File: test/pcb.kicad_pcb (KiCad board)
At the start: 2 copper layers, 98 x 120 mm, 25 parts, among them M1 RasPiPico, SW1 SW_Push, SW10 SW_Push, SW11 SW_Push, SW12 SW_Push, SW13 SW_Push, SW14 SW_Push, SW15 SW_Push, SW16 SW_Push, SW17 SW_Push, SW18 SW_Push, SW19 SW_Push, SW2 SW_Push, SW20 SW_Push, SW21 SW_Push, SW22 SW_Push, SW3 SW_Push, SW4 SW_Push, SW5 SW_Push, SW7 SW_Push, SW8 SW_Push, SW9 SW_Push

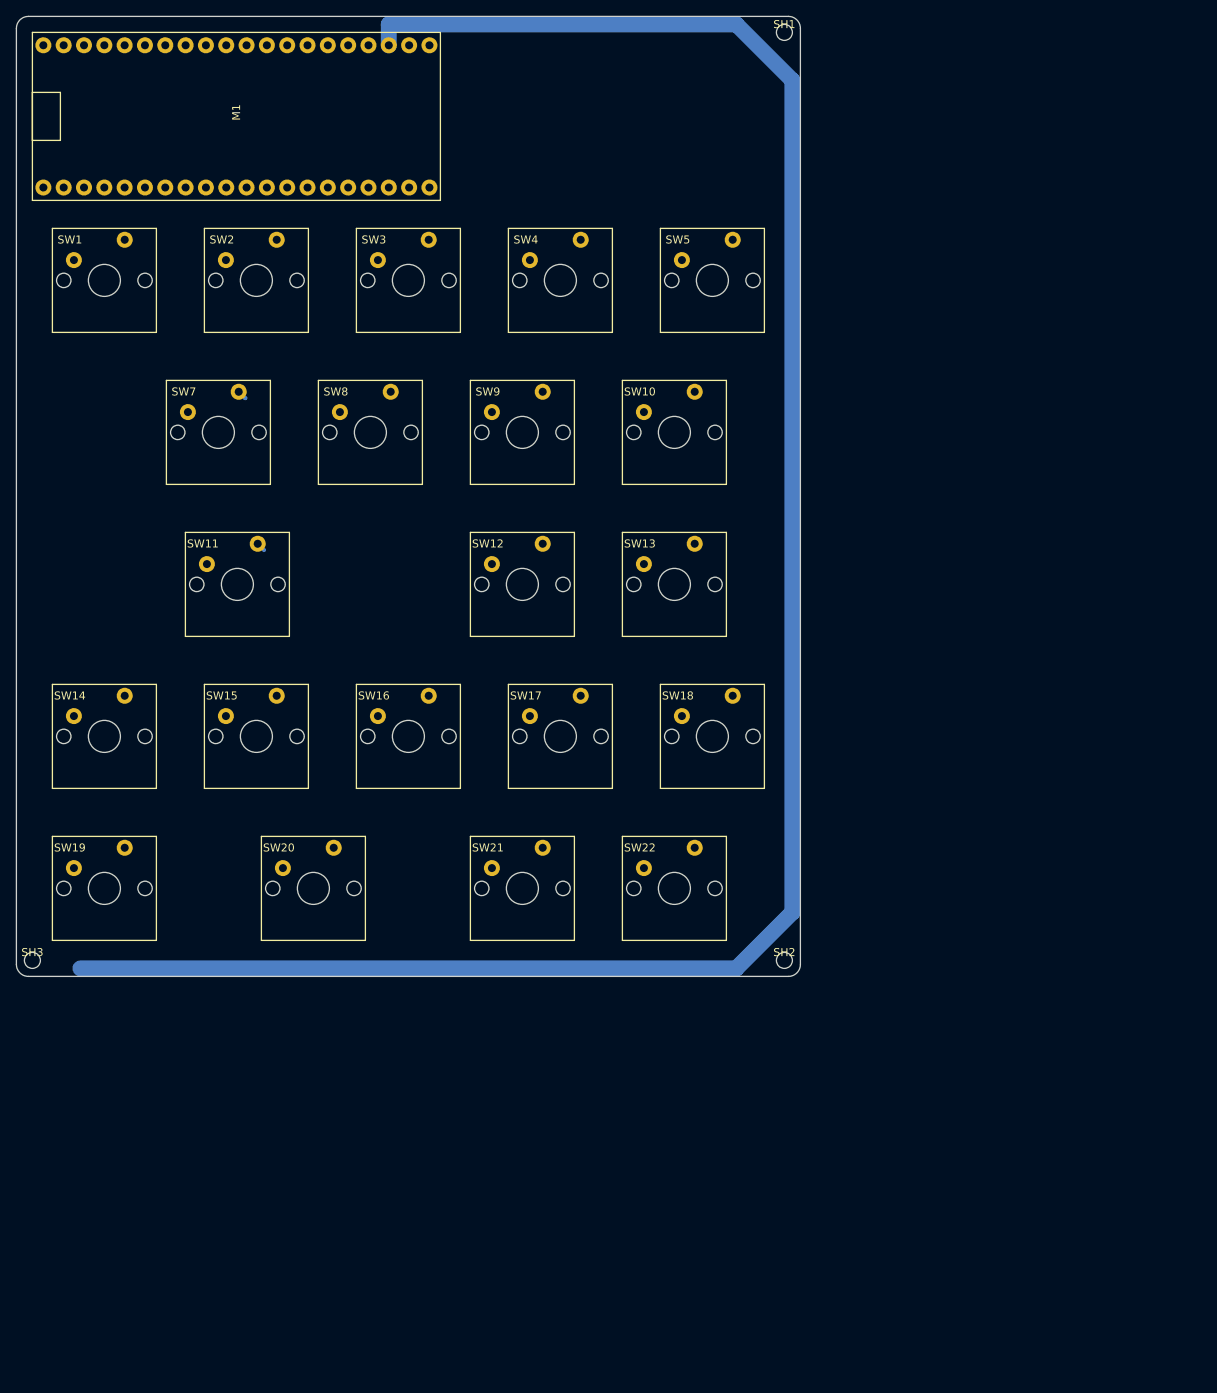
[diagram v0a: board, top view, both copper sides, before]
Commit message: fix file size 0
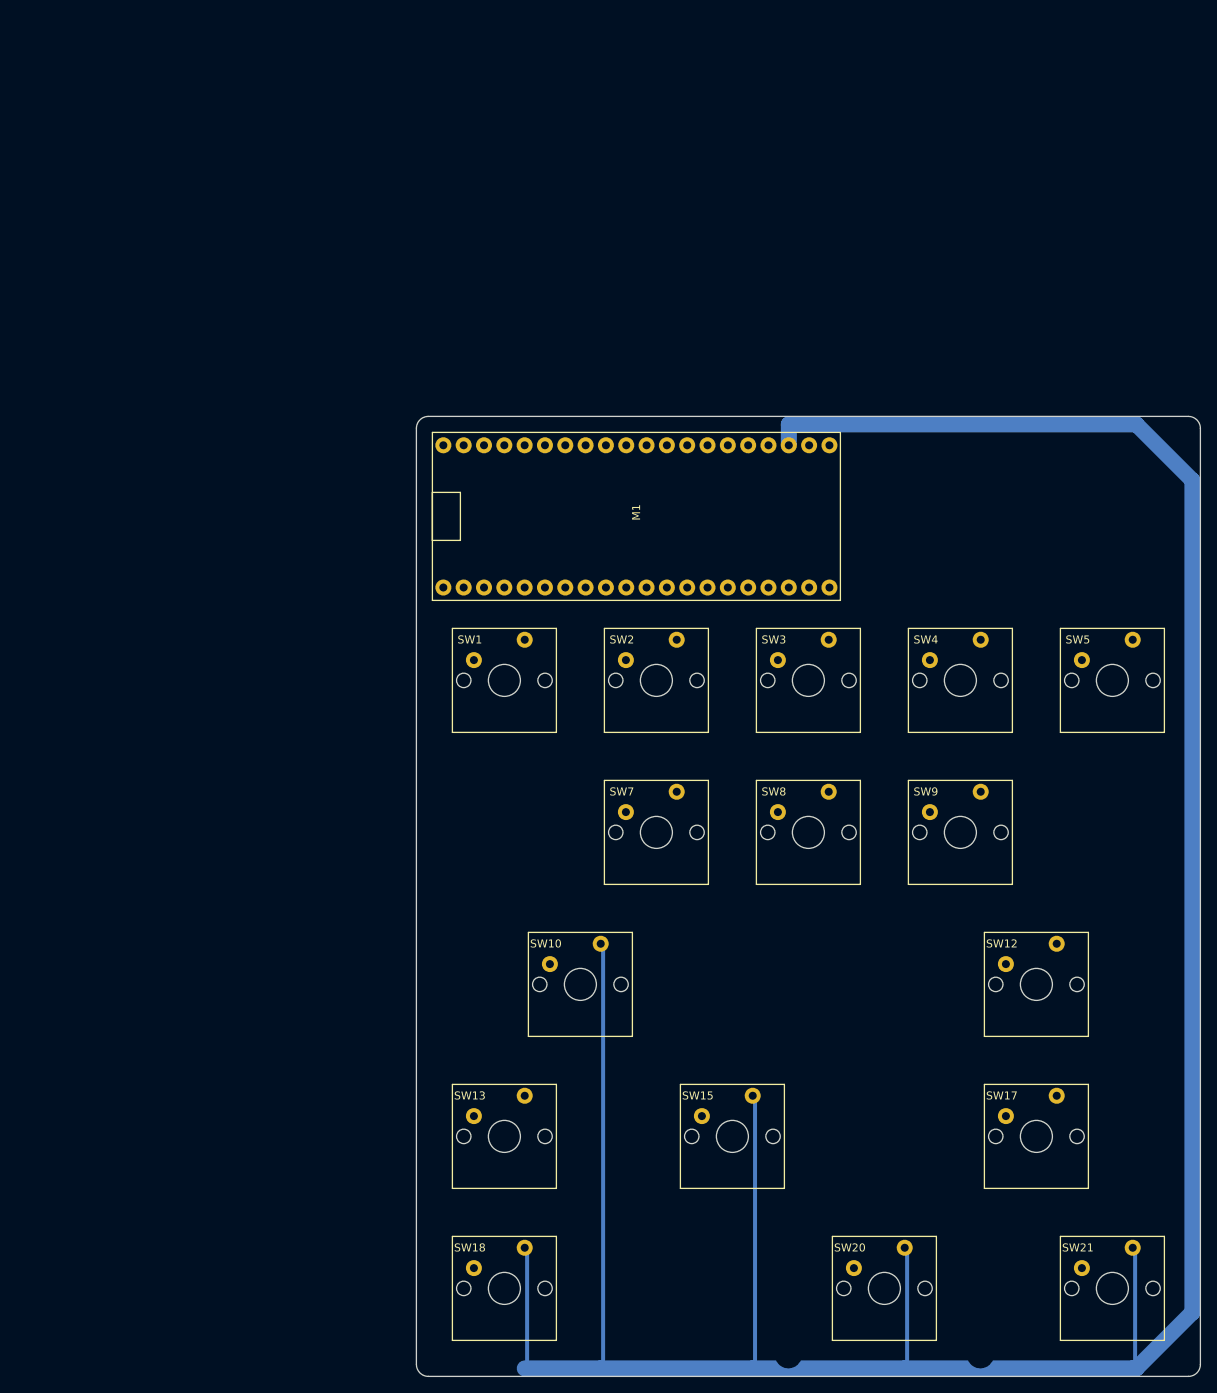
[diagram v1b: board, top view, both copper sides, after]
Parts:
- removed the M1 at (27.5, 12.5)
- removed SH2, SH3: SCREW_HOLE, footprint:screwhole
- removed SW11: SW_Push, footprint:keyswitch-with-stabilizer
- removed SW14, SW16, SW19, SW22: SW_Push, footprint:keyswitch
- M1: renamed from SH1; value SCREW_HOLE -> RasPiPico; footprint footprint:screwhole -> footprint:pipico
- SW10, SW20: footprint footprint:keyswitch -> footprint:keyswitch-with-stabilizer
- moved SW21 89.1 mm to (137.0, 159.0)
- moved SW20 87.1 mm to (108.5, 159.0)
- moved SW12 81.4 mm to (127.5, 121.0)
- moved SW15 77.7 mm to (89.5, 140.0)
- moved SW17 77.7 mm to (127.5, 140.0)
- moved SW7 74.1 mm to (80.0, 102.0)
- moved SW8 74.1 mm to (99.0, 102.0)
- moved SW9 74.1 mm to (118.0, 102.0)
- moved SW18 73.7 mm to (61.0, 159.0)
- moved SW13 72.2 mm to (61.0, 140.0)
- moved SW1 70.7 mm to (61.0, 83.0)
- moved SW2 70.7 mm to (80.0, 83.0)
- moved SW3 70.7 mm to (99.0, 83.0)
- moved SW4 70.7 mm to (118.0, 83.0)
- moved SW5 70.7 mm to (137.0, 83.0)
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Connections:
- SW1 pad 1: GP4 -> GP2
- SW10 pad 1: GP17 -> GP6
- SW12 pad 1: GP26 -> GP18
- SW13 pad 1: GP18 -> GP1
- SW15 pad 1: GP6 -> GP11
- SW17 pad 1: GP27 -> GP19
- SW18 pad 1: GP19 -> GP0
- SW2 pad 1: GP9 -> GP8
- SW20 pad 1: GP5 -> GP28
- SW21 pad 1: GP28 -> GP20
- SW3 pad 1: GP14 -> GP13
- SW4 pad 1: GP21 -> GP26
- SW5 pad 1: GP16 -> GP17
- SW7 pad 1: GP8 -> GP7
- SW8 pad 1: GP13 -> GP12
- SW9 pad 1: GP22 -> GP27
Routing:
- net GND4: track 264.3 -> 380.5 mm
